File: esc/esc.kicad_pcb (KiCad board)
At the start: 2 copper layers, 6 parts, among them IC1 IR2103STRPBF, Q1 SiR180DP-T1-RE3, U1 STM32G474RETx, Y1 NX2016SA-24M-EXS00A-CS08891

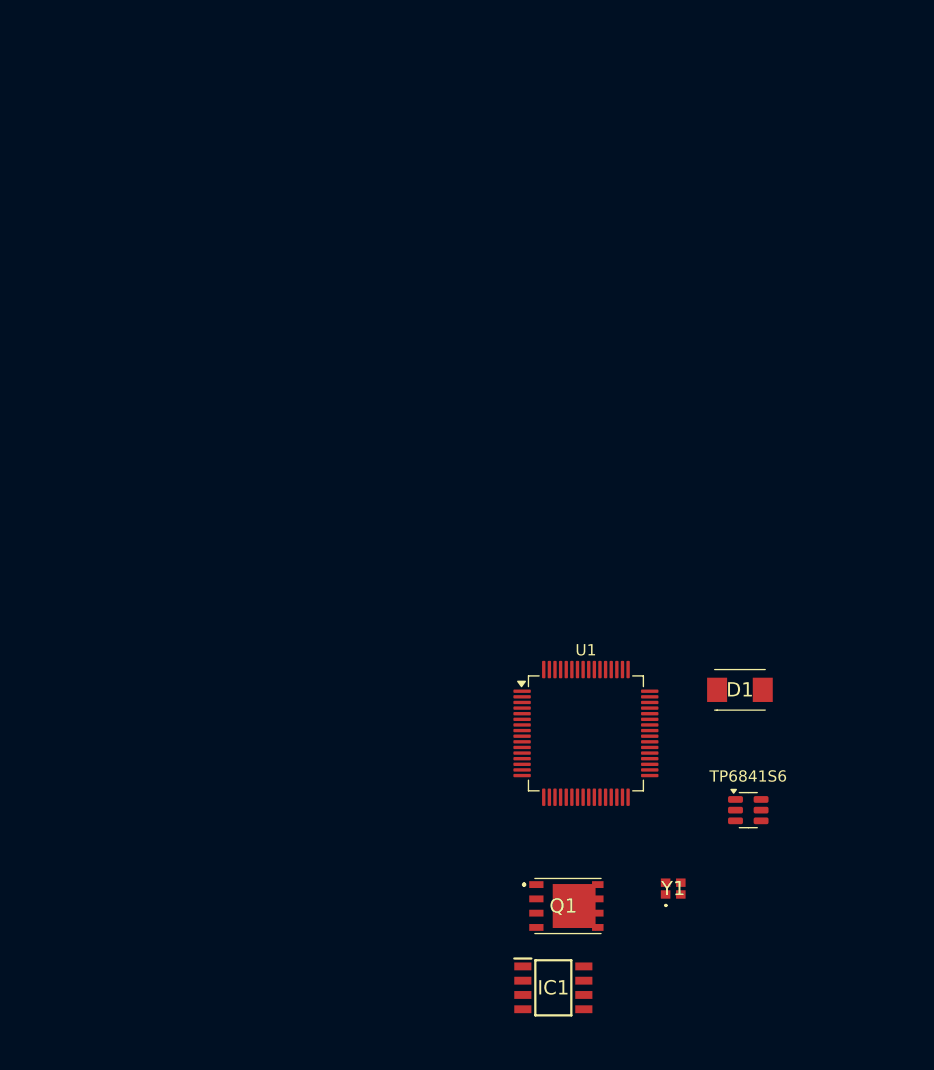
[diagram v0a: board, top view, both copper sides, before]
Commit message: full layout
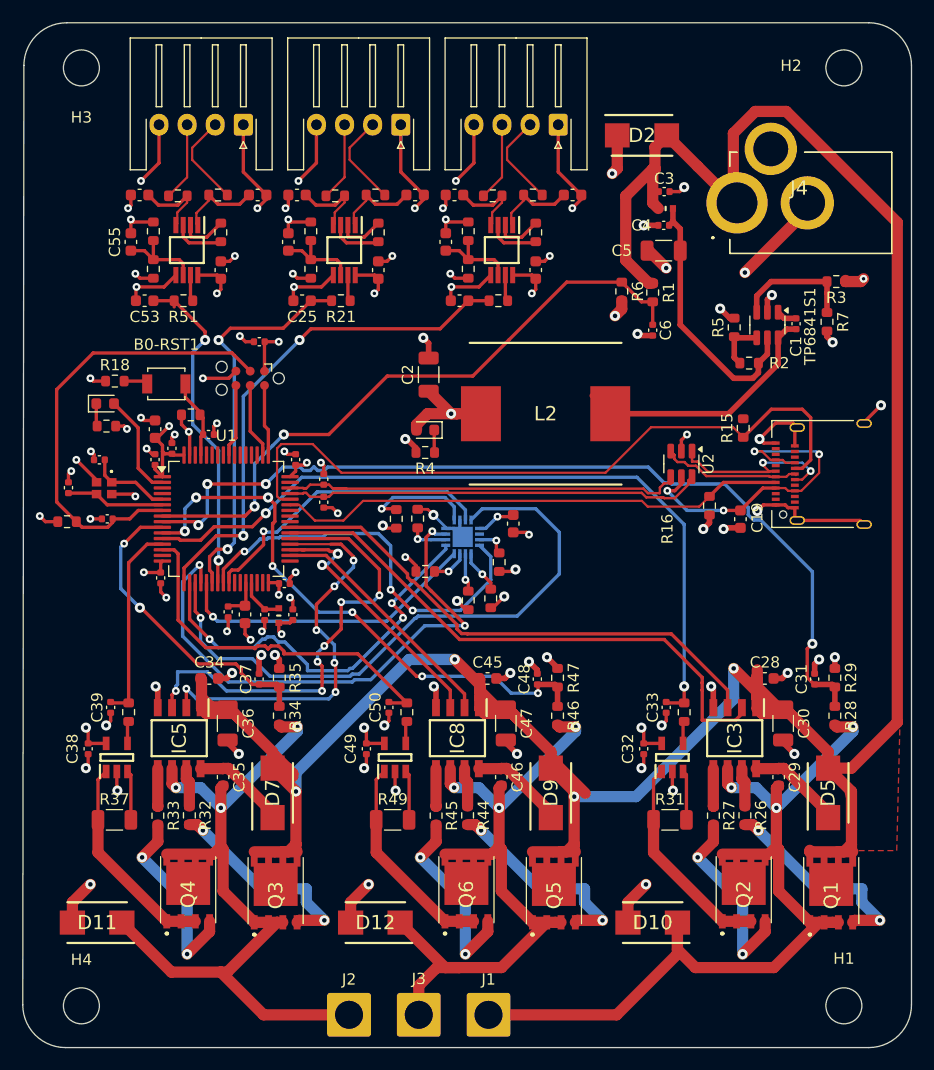
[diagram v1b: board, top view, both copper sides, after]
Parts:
- removed TP6841S6: ~, Package_TO_SOT_SMD:SOT-23-6
- added B0-RST1: SW_Push, Button_Switch_SMD:SW_SPST_B3U-1000P, F.Cu at (113.8, 81.1)
- added C1: 100n, Capacitor_SMD:C_0402_1005Metric, F.Cu at (169.8, 75.8)
- added C10: 100n, Capacitor_SMD:C_0402_1005Metric, F.Cu at (113.2, 98.3)
- added C11: 100n, Capacitor_SMD:C_0402_1005Metric, F.Cu at (125.2, 87.8)
- added C12: 100n, Capacitor_SMD:C_0402_1005Metric, F.Cu at (124.2, 98.8)
- added C13: 1u, Capacitor_SMD:C_0603_1608Metric, F.Cu at (144.6, 93.5)
- added C14: 100n, Capacitor_SMD:C_0402_1005Metric, F.Cu at (108.5, 93.1)
- added C15: 100n, Capacitor_SMD:C_0402_1005Metric, F.Cu at (122.5, 101.6)
- added C16: 100n, Capacitor_SMD:C_0402_1005Metric, F.Cu at (112.8, 87.8)
- added C17: 100n, Capacitor_SMD:C_0402_1005Metric, F.Cu at (127.8, 89.6)
- added C18: 100n, Capacitor_SMD:C_0402_1005Metric, F.Cu at (127.8, 91.6)
- added C19: 1u, Capacitor_SMD:C_0603_1608Metric, F.Cu at (164.8, 93.1)
- added C2: 47u, Capacitor_SMD:C_1206_3216Metric, F.Cu at (137.1, 80.3)
- added C20: 100n, Capacitor_SMD:C_0402_1005Metric, F.Cu at (117.5, 85.6)
- added C21: 6p8, Capacitor_SMD:C_0402_1005Metric, F.Cu at (105.0, 90.3)
- added C22: 6p8, Capacitor_SMD:C_0402_1005Metric, F.Cu at (107.8, 87.8)
- added C23: 0u1, Capacitor_SMD:C_0603_1608Metric, F.Cu at (132.6, 71.0)
- added C24: 0u1, Capacitor_SMD:C_0603_1608Metric, F.Cu at (135.9, 64.3)
- added C25: 0u1, Capacitor_SMD:C_0603_1608Metric, F.Cu at (125.8, 73.7)
- added C26: 0u1, Capacitor_SMD:C_0603_1608Metric, F.Cu at (125.4, 64.3)
- added C27: 0u1, Capacitor_SMD:C_0603_1608Metric, F.Cu at (124.6, 68.5)
- added C28: 1u, Capacitor_SMD:C_0603_1608Metric, F.Cu at (167.0, 107.3)
- added C29: 1u, Capacitor_SMD:C_0603_1608Metric, F.Cu at (168.2, 116.1)
- added C3: 100n, Capacitor_SMD:C_0402_1005Metric, F.Cu at (158.0, 64.0)
- added C30: 47u, Capacitor_SMD:C_1206_3216Metric, F.Cu at (168.6, 111.3)
- added C31: 10n, Capacitor_SMD:C_0402_1005Metric, F.Cu at (171.4, 107.3)
- added C32: 100n, Capacitor_SMD:C_0402_1005Metric, F.Cu at (156.2, 113.5)
- added C33: 1n, Capacitor_SMD:C_0402_1005Metric, F.Cu at (158.2, 109.9)
- added C34: 1u, Capacitor_SMD:C_0603_1608Metric, F.Cu at (117.6, 107.3)
- added C35: 1u, Capacitor_SMD:C_0603_1608Metric, F.Cu at (118.8, 116.1)
- added C36: 47u, Capacitor_SMD:C_1206_3216Metric, F.Cu at (119.2, 111.3)
- added C37: 10n, Capacitor_SMD:C_0402_1005Metric, F.Cu at (122.0, 107.3)
- added C38: 100n, Capacitor_SMD:C_0402_1005Metric, F.Cu at (106.8, 113.5)
- added C39: 1n, Capacitor_SMD:C_0402_1005Metric, F.Cu at (108.8, 109.9)
- added C4: 100n, Capacitor_SMD:C_0402_1005Metric, F.Cu at (158.0, 67.0)
- added C40: 0u1, Capacitor_SMD:C_0603_1608Metric, F.Cu at (146.6, 71.0)
- added C41: 0u1, Capacitor_SMD:C_0603_1608Metric, F.Cu at (149.9, 64.3)
- added C42: 0u1, Capacitor_SMD:C_0603_1608Metric, F.Cu at (139.8, 73.7)
- added C43: 0u1, Capacitor_SMD:C_0603_1608Metric, F.Cu at (139.4, 64.3)
- added C44: 0u1, Capacitor_SMD:C_0603_1608Metric, F.Cu at (138.6, 68.5)
- added C45: 1u, Capacitor_SMD:C_0603_1608Metric, F.Cu at (142.3, 107.3)
- added C46: 1u, Capacitor_SMD:C_0603_1608Metric, F.Cu at (143.5, 116.1)
- added C47: 47u, Capacitor_SMD:C_1206_3216Metric, F.Cu at (143.9, 111.3)
- added C48: 10n, Capacitor_SMD:C_0402_1005Metric, F.Cu at (146.7, 107.3)
- added C49: 100n, Capacitor_SMD:C_0402_1005Metric, F.Cu at (131.5, 113.5)
- added C5: 47u, Capacitor_SMD:C_1206_3216Metric, F.Cu at (158.0, 69.2)
- added C50: 1n, Capacitor_SMD:C_0402_1005Metric, F.Cu at (133.5, 109.9)
- added C51: 0u1, Capacitor_SMD:C_0603_1608Metric, F.Cu at (118.6, 71.0)
- added C52: 0u1, Capacitor_SMD:C_0603_1608Metric, F.Cu at (121.9, 64.3)
- added C53: 0u1, Capacitor_SMD:C_0603_1608Metric, F.Cu at (111.8, 73.7)
- added C54: 0u1, Capacitor_SMD:C_0603_1608Metric, F.Cu at (111.4, 64.3)
- added C55: 0u1, Capacitor_SMD:C_0603_1608Metric, F.Cu at (110.6, 68.5)
- added C56: 100n, Capacitor_SMD:C_0402_1005Metric, F.Cu at (119.2, 101.4)
- added C57: 1u, Capacitor_SMD:C_0603_1608Metric, F.Cu at (120.8, 101.6)
- added C58: 100n, Capacitor_SMD:C_0402_1005Metric, F.Cu at (122.0, 77.3)
- added C6: 10n, Capacitor_SMD:C_0402_1005Metric, F.Cu at (157.0, 76.3)
- added C7: 4u7, Capacitor_SMD:C_0603_1608Metric, F.Cu at (112.8, 85.1)
- added C8: 100n, Capacitor_SMD:C_0402_1005Metric, F.Cu at (125.0, 101.6)
- added C9: 100n, Capacitor_SMD:C_0402_1005Metric, F.Cu at (114.2, 86.8)
- added D10: SMBJ18A-13-F, SamacSys_Parts:DIOM5336X250N, F.Cu at (157.0, 129.0)
- added D11: SMBJ18A-13-F, SamacSys_Parts:DIOM5336X250N, F.Cu at (107.6, 129.0)
- added D12: SMBJ18A-13-F, SamacSys_Parts:DIOM5336X250N, F.Cu at (132.3, 129.0)
- added D2: SMBJ18A, SamacSys_Parts:DIOM5436X244N, F.Cu at (156.1, 59.0)
- added D3: LED, LED_SMD:LED_0603_1608Metric, F.Cu at (108.3, 82.8)
- added D5: SMBJ18A-13-F, SamacSys_Parts:DIOM5336X250N, F.Cu at (172.6, 117.5)
- added D7: SMBJ18A-13-F, SamacSys_Parts:DIOM5336X250N, F.Cu at (123.2, 117.5)
- added D9: SMBJ18A-13-F, SamacSys_Parts:DIOM5336X250N, F.Cu at (147.9, 117.5)
- added FB1: MMZ1005F181ETD25, SamacSys_Parts:BEADC1005X55N, F.Cu at (158.2, 65.5)
- added FB2: MMZ1005F181ETD25, SamacSys_Parts:BEADC1005X55N, F.Cu at (123.8, 101.7)
- added FSENS1: Conn_01x04_Socket, Connector_JST:JST_XH_S4B-XH-A-1_1x04_P2.50mm_Horizontal, F.Cu at (134.6, 58.1)
- added FSENS2: Conn_01x04_Socket, Connector_JST:JST_XH_S4B-XH-A-1_1x04_P2.50mm_Horizontal, F.Cu at (148.6, 58.0)
- added FSENS3: Conn_01x04_Socket, Connector_JST:JST_XH_S4B-XH-A-1_1x04_P2.50mm_Horizontal, F.Cu at (120.6, 58.1)
- added H1: MountingHole, MountingHole:MountingHole_3.2mm_M3, F.Cu at (174.0, 136.4)
- added H2: MountingHole, MountingHole:MountingHole_3.2mm_M3, F.Cu at (174.0, 53.0)
- added H3: MountingHole, MountingHole:MountingHole_3.2mm_M3, F.Cu at (106.2, 53.0)
- added H4: MountingHole, MountingHole:MountingHole_3.2mm_M3, F.Cu at (106.2, 136.4)
- added IC10: AD8221ARMZ, SamacSys_Parts:SOP65P490X110-8N, F.Cu at (115.6, 69.2)
- added IC2: AD8221ARMZ, SamacSys_Parts:SOP65P490X110-8N, F.Cu at (129.6, 69.2)
- added IC3: IR2103STRPBF, SamacSys_Parts:SOIC127P600X175-8N, F.Cu at (164.3, 112.6)
- added IC4: INA180A3IDBVT, SamacSys_Parts:SOT95P280X145-5N, F.Cu at (158.8, 114.3)
- added IC5: IR2103STRPBF, SamacSys_Parts:SOIC127P600X175-8N, F.Cu at (114.9, 112.6)
- added IC6: INA180A3IDBVT, SamacSys_Parts:SOT95P280X145-5N, F.Cu at (109.3, 114.3)
- added IC7: AD8221ARMZ, SamacSys_Parts:SOP65P490X110-8N, F.Cu at (143.6, 69.2)
- added IC8: IR2103STRPBF, SamacSys_Parts:SOIC127P600X175-8N, F.Cu at (139.6, 112.6)
- added IC9: INA180A3IDBVT, SamacSys_Parts:SOT95P280X145-5N, F.Cu at (134.1, 114.3)
- added J1: Conn_A, Connector_Wire:SolderWire-2sqmm_1x01_D2mm_OD3.9mm, F.Cu at (142.4, 137.2)
- added J2: Conn_B, Connector_Wire:SolderWire-2sqmm_1x01_D2mm_OD3.9mm, F.Cu at (130.0, 137.2)
- added J3: Conn_C, Connector_Wire:SolderWire-2sqmm_1x01_D2mm_OD3.9mm, F.Cu at (136.2, 137.2)
- added J4: KLDHCX-0202-BC-1, SamacSys_Parts:KLDHCX0202BC1, F.Cu at (164.5, 65.0)
- added J5: USB_C_Receptacle_USB2.0_14P, Connector_USB:USB_C_Receptacle_Amphenol_12401610E4-2A, F.Cu at (173.0, 89.1)
- added J6: SWD_TagConnect_TC2030-NL, Connector:Tag-Connect_TC2030-IDC-NL_2x03_P1.27mm_Vertical, F.Cu at (121.2, 80.6)
- added L2: PA4343.682ANLT, SamacSys_Parts:INDPM135126X650N, F.Cu at (147.5, 83.8)
- added Q2: SiR182DP-T1-RE3, SamacSys_Parts:SI7141DPT1GE3, F.Cu at (165.1, 126.1)
- added Q3: SiR182DP-T1-RE3, SamacSys_Parts:SI7141DPT1GE3, F.Cu at (123.5, 126.2)
- added Q4: SiR182DP-T1-RE3, SamacSys_Parts:SI7141DPT1GE3, F.Cu at (115.7, 126.1)
- added Q5: SiR182DP-T1-RE3, SamacSys_Parts:SI7141DPT1GE3, F.Cu at (148.2, 126.2)
- added Q6: SiR182DP-T1-RE3, SamacSys_Parts:SI7141DPT1GE3, F.Cu at (140.4, 126.1)
- added R1: 4k7, Resistor_SMD:R_0603_1608Metric, F.Cu at (157.0, 73.0)
- added R10: 10k, Resistor_SMD:R_0603_1608Metric, F.Cu at (142.6, 100.2)
- added R11: 10k, Resistor_SMD:R_0603_1608Metric, F.Cu at (140.6, 100.3)
- added R12: 10k, Resistor_SMD:R_0603_1608Metric, F.Cu at (136.8, 97.8)
- added R13: 10k, Resistor_SMD:R_0603_1608Metric, F.Cu at (134.2, 93.1)
- added R14: 10k, Resistor_SMD:R_0603_1608Metric, F.Cu at (136.1, 93.1)
- added R15: 5k1, Resistor_SMD:R_0603_1608Metric, F.Cu at (165.1, 85.0)
- added R16: 5k1, Resistor_SMD:R_0603_1608Metric, F.Cu at (162.1, 91.9)
- added R17: 1k, Resistor_SMD:R_0603_1608Metric, F.Cu at (108.4, 84.8)
- added R18: 100R, Resistor_SMD:R_0603_1608Metric, F.Cu at (109.2, 80.8)
- added R19: 10k, Resistor_SMD:R_0603_1608Metric, F.Cu at (115.9, 83.8)
- added R2: 110k, Resistor_SMD:R_0603_1608Metric, F.Cu at (165.6, 79.2)
- added R20: 4k02, Resistor_SMD:R_0603_1608Metric, F.Cu at (132.3, 64.3)
- added R21: 1k0, Resistor_SMD:R_0603_1608Metric, F.Cu at (129.3, 73.7)
- added R22: 180, Resistor_SMD:R_0603_1608Metric, F.Cu at (132.6, 67.6)
- added R23: 4k02, Resistor_SMD:R_0603_1608Metric, F.Cu at (128.8, 64.4)
- added R24: 10k, Resistor_SMD:R_0603_1608Metric, F.Cu at (126.6, 70.9)
- added R25: 10k, Resistor_SMD:R_0603_1608Metric, F.Cu at (126.6, 67.5)
- added R26: 100R, Resistor_SMD:R_0603_1608Metric, F.Cu at (165.2, 119.5)
- added R27: 100R, Resistor_SMD:R_0603_1608Metric, F.Cu at (162.4, 119.5)
- added R28: 4k7, Resistor_SMD:R_0603_1608Metric, F.Cu at (173.2, 110.6)
- added R29: 1k, Resistor_SMD:R_0603_1608Metric, F.Cu at (173.2, 107.2)
- added R3: 75k, Resistor_SMD:R_0603_1608Metric, F.Cu at (173.3, 72.0)
- added R30: 1k, Resistor_SMD:R_0603_1608Metric, F.Cu at (159.8, 110.3)
- added R31: 2mR, Resistor_SMD:R_1206_3216Metric, F.Cu at (158.5, 119.9)
- added R32: 100R, Resistor_SMD:R_0603_1608Metric, F.Cu at (115.8, 119.5)
- added R33: 100R, Resistor_SMD:R_0603_1608Metric, F.Cu at (113.0, 119.5)
- added R34: 4k7, Resistor_SMD:R_0603_1608Metric, F.Cu at (123.8, 110.6)
- added R35: 1k, Resistor_SMD:R_0603_1608Metric, F.Cu at (123.8, 107.2)
- added R36: 1k, Resistor_SMD:R_0603_1608Metric, F.Cu at (110.4, 110.3)
- added R37: 2mR, Resistor_SMD:R_1206_3216Metric, F.Cu at (109.1, 119.9)
- added R38: 4k02, Resistor_SMD:R_0603_1608Metric, F.Cu at (146.4, 64.3)
- added R39: 1k0, Resistor_SMD:R_0603_1608Metric, F.Cu at (143.3, 73.7)
- added R4: 1k, Resistor_SMD:R_0603_1608Metric, F.Cu at (136.8, 87.2)
- added R40: 180, Resistor_SMD:R_0603_1608Metric, F.Cu at (146.6, 67.6)
- added R41: 4k02, Resistor_SMD:R_0603_1608Metric, F.Cu at (142.8, 64.4)
- added R42: 10k, Resistor_SMD:R_0603_1608Metric, F.Cu at (140.6, 70.9)
- added R43: 10k, Resistor_SMD:R_0603_1608Metric, F.Cu at (140.6, 67.5)
- added R44: 100R, Resistor_SMD:R_0603_1608Metric, F.Cu at (140.5, 119.5)
- added R45: 100R, Resistor_SMD:R_0603_1608Metric, F.Cu at (137.7, 119.5)
- added R46: 4k7, Resistor_SMD:R_0603_1608Metric, F.Cu at (148.5, 110.6)
- added R47: 1k, Resistor_SMD:R_0603_1608Metric, F.Cu at (148.5, 107.2)
- added R48: 1k, Resistor_SMD:R_0603_1608Metric, F.Cu at (135.1, 110.3)
- added R49: 2mR, Resistor_SMD:R_1206_3216Metric, F.Cu at (133.9, 119.9)
- added R5: 12k, Resistor_SMD:R_0603_1608Metric, F.Cu at (164.2, 76.1)
- added R50: 4k02, Resistor_SMD:R_0603_1608Metric, F.Cu at (118.4, 64.3)
- added R51: 1k0, Resistor_SMD:R_0603_1608Metric, F.Cu at (115.3, 73.7)
- added R52: 180, Resistor_SMD:R_0603_1608Metric, F.Cu at (118.6, 67.6)
- added R53: 4k02, Resistor_SMD:R_0603_1608Metric, F.Cu at (114.8, 64.4)
- added R54: 10k, Resistor_SMD:R_0603_1608Metric, F.Cu at (112.6, 70.9)
- added R55: 10k, Resistor_SMD:R_0603_1608Metric, F.Cu at (112.6, 67.5)
- added R6: 1k, Resistor_SMD:R_0603_1608Metric, F.Cu at (154.2, 72.9)
- added R7: 24k, Resistor_SMD:R_0603_1608Metric, F.Cu at (172.5, 75.6)
- added R8: 10k, Resistor_SMD:R_0603_1608Metric, F.Cu at (143.3, 97.0)
- added R9: 10k, Resistor_SMD:R_0603_1608Metric, F.Cu at (104.9, 93.3)
- added TP6841S1: ~, Package_TO_SOT_SMD:SOT-23-6, F.Cu at (167.2, 75.9)
- added U2: USBLC6-2SC6, Package_TO_SOT_SMD:SOT-23-6, F.Cu at (159.6, 88.2)
- D1: value SMBJ18A -> LED; footprint SamacSys_Parts:SMBJ18A -> LED_SMD:LED_0603_1608Metric
- IC1: value IR2103STRPBF -> MA702GQ-P; footprint SamacSys_Parts:SOIC127P600X175-8N -> SamacSys_Parts:QFN50P300X300X100-17N-D; moved to B.Cu
- Q1: value SiR180DP-T1-RE3 -> SiR182DP-T1-RE3
- moved Y1 61.9 mm to (108.2, 90.4), turned to 180 degrees
- moved IC1 40.9 mm to (140.1, 94.7), turned to 90 degrees
- moved U1 37.2 mm to (119.1, 93.1)
- moved D1 36.3 mm to (136.8, 85.2), turned to 180 degrees
- moved Q1 23.4 mm to (172.9, 126.2), turned to 90 degrees
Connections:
- D1 pad 1: VCC -> /LED_PWR_K
- D1 pad 2: GND -> 3V3
- IC1 pad 1: unconnected-(IC1-VCC-Pad1) -> /SSD
- IC1 pad 2: unconnected-(IC1-HIN-Pad2) -> /MG_A
- IC1 pad 3: unconnected-(IC1-~{LIN}-Pad3) -> /MG_Z
- IC1 pad 4: unconnected-(IC1-COM-Pad4) -> /MGH_SPI1_MOSI
- IC1 pad 5: unconnected-(IC1-LO-Pad5) -> /MGH_SPI1_NSS
- IC1 pad 6: unconnected-(IC1-VS-Pad6) -> /MG_B
- IC1 pad 7: unconnected-(IC1-HO-Pad7) -> /MGH_SPI1_MISO
- IC1 pad 8: unconnected-(IC1-VB-Pad8) -> GND
- Q1 pad 1: unconnected-(Q1-S_1-Pad1) -> /VPH_A
- Q1 pad 2: unconnected-(Q1-S_2-Pad2) -> /VPH_A
- Q1 pad 3: unconnected-(Q1-S_3-Pad3) -> /VPH_A
- Q1 pad 4: unconnected-(Q1-G-Pad4) -> /Phase_A/VHO_R
- Q1 pad 5: unconnected-(Q1-D_1-Pad5) -> VCC
- Q1 pad 6: unconnected-(Q1-D_2-Pad6) -> VCC
- Q1 pad 7: unconnected-(Q1-D_3-Pad7) -> VCC
- Q1 pad 8: unconnected-(Q1-D_4-Pad8) -> VCC
- U1 pad 10: VISENSE_C -> /VSENSE_B
- U1 pad 11: unconnected-(U1-PC3-Pad11) -> /VSENSE_C
- U1 pad 12: VISENSE_A -> /VISENSE_A
- U1 pad 13: unconnected-(U1-PA1-Pad13) -> /VISENSE_B
- U1 pad 14: VISENSE_B -> /VISENSE_C
- U1 pad 17: unconnected-(U1-PA3-Pad17) -> /SG_1
- U1 pad 18: unconnected-(U1-PA4-Pad18) -> /MGH_SPI1_NSS
- U1 pad 19: unconnected-(U1-PA5-Pad19) -> /MGH_SPI1_SCK
- U1 pad 2: Net-(D3-A) -> /LED_MCU
- U1 pad 20: unconnected-(U1-PA6-Pad20) -> /MGH_SPI1_MISO
- U1 pad 21: unconnected-(U1-PA7-Pad21) -> /MGH_SPI1_MOSI
- U1 pad 22: unconnected-(U1-PC4-Pad22) -> /SG_2
- U1 pad 23: unconnected-(U1-PC5-Pad23) -> /SG_3
- U1 pad 24: unconnected-(U1-PB0-Pad24) -> /MGH_MGH
- U1 pad 25: unconnected-(U1-PB1-Pad25) -> /MGH_MGL
- U1 pad 28: 3V3 -> /3V3_Filt
- U1 pad 29: 3V3 -> /3V3_Filt
- U1 pad 34: unconnected-(U1-PB12-Pad34) -> /HIN_C
- U1 pad 35: unconnected-(U1-PB13-Pad35) -> /LIN_C
- U1 pad 36: unconnected-(U1-PB14-Pad36) -> /HIN_B
- U1 pad 37: unconnected-(U1-PB15-Pad37) -> /LIN_B
- U1 pad 38: unconnected-(U1-PC6-Pad38) -> /HIN_A
- U1 pad 39: unconnected-(U1-PC7-Pad39) -> /LIN_A
- U1 pad 40: I2C_SCL -> unconnected-(U1-PC8-Pad40)
- U1 pad 41: I2C_SCA -> unconnected-(U1-PC9-Pad41)
- U1 pad 42: HIN_A -> unconnected-(U1-PA8-Pad42)
- U1 pad 43: HIN_B -> /USB_DBCC2
- U1 pad 44: HIN_C -> /USB_DBCC1
- U1 pad 45: unconnected-(U1-PA11-Pad45) -> /USB_D-
- U1 pad 46: unconnected-(U1-PA12-Pad46) -> /USB_D+
- U1 pad 49: unconnected-(U1-PA13-Pad49) -> /MCU_SWDIO
- U1 pad 50: unconnected-(U1-PA14-Pad50) -> /MCU_SWCLK
- U1 pad 56: unconnected-(U1-PB3-Pad56) -> /MCU_SWO
- U1 pad 61: Net-(U1-PB8) -> /BOOT0
- U1 pad 7: Net-(U1-PG10) -> /MCU_NRST
- U1 pad 8: VCC_SENSE -> /VCC_SENSE
- U1 pad 9: unconnected-(U1-PC1-Pad9) -> /VSENSE_A
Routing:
- net VCC: track 0.00 -> 272.1 mm, vias 0 -> 4
- net GND: track 0.00 -> 214.5 mm, vias 0 -> 89
- net 3V3: track 0.00 -> 83.0 mm, vias 0 -> 23
- net /VSENSE_A: track 0.00 -> 80.6 mm, vias 0 -> 4
- net /VPH_A: track 0.00 -> 78.5 mm, vias 0 -> 3
- net /VPH_B: track 0.00 -> 69.8 mm, vias 0 -> 3
- net /VISENSE_A: track 0.00 -> 68.0 mm, vias 0 -> 2
- net /USB_DBCC1: track 0.00 -> 63.1 mm
- net /VPH_C: track 0.00 -> 62.6 mm, vias 0 -> 3
- net /VCC_SENSE: track 0.00 -> 57.2 mm, vias 0 -> 2
- net /MGH_SPI1_SCK: track 0.00 -> 55.2 mm, vias 0 -> 1
- net /VSENSE_C: track 0.00 -> 51.0 mm, vias 0 -> 7
- net /HIN_A: track 0.00 -> 50.1 mm
- net /MGH_SPI1_MISO: track 0.00 -> 48.8 mm, vias 0 -> 3
- net /LIN_A: track 0.00 -> 46.9 mm
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- added copper zone on In2.Cu, net 3V3
- added copper zone on In1.Cu, net GND
- added copper zone on F.Cu, net VCC
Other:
- board outline added: 79 x 91.1 mm
- copper layers 2 -> 4
